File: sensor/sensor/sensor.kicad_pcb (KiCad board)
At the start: 2 copper layers, 39 parts, among them J1 RJ12_Shielded, J2 Conn_01x04, J3 Conn_01x06, J4 Conn_01x05, J5 Conn_01x05, J8 RJ12_Shielded, J9 Conn_01x06, SW5 SW_Coded_SH-7050, U1 PCA9615DP, U2 LTC4316, U5 TPS73101DBV

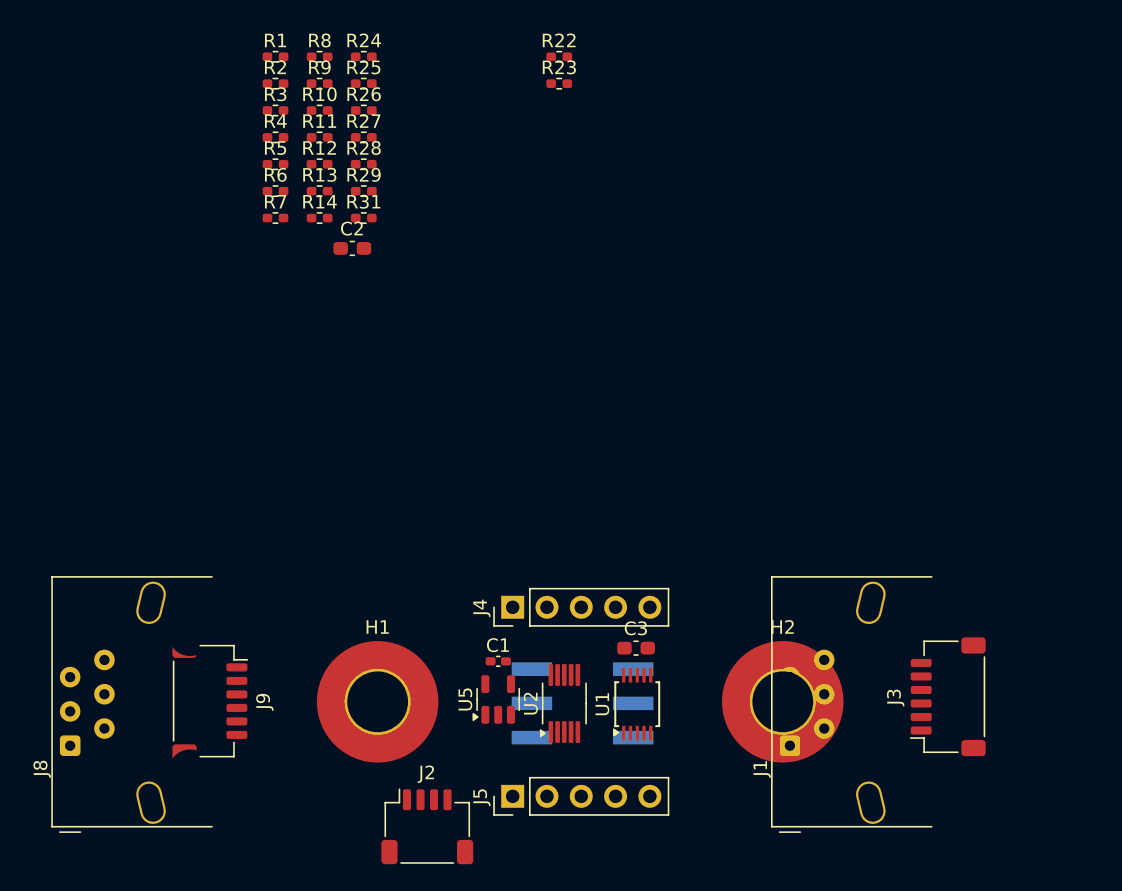
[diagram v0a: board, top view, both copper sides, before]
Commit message: finished main sensor board
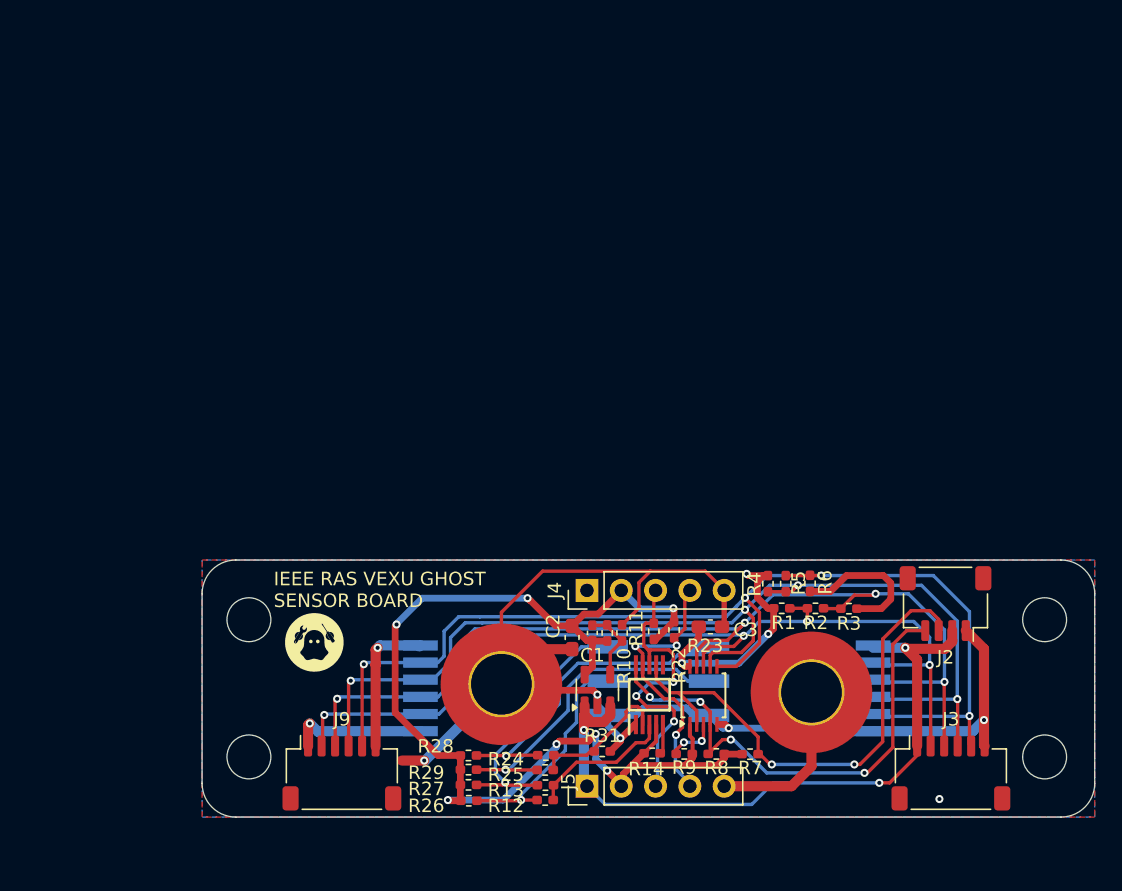
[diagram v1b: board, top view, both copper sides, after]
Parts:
- removed J8: RJ12_Shielded, RJ12_Pin_Connector:RJ12_Pin_Connector
- removed U2: LTC4316, Package_SO:MSOP-10_3x3mm_P0.5mm
- added G***: LOGO, LOGO, F.Cu at (110.3, 105.6)
- added G***: LOGO, LOGO, B.Cu at (110.7, 102.8)
- added G***: LOGO, LOGO, B.Cu at (114.8, 101.9)
- added IC1: LTC4316CMS#TRPBF, LTC4316CMS:SOP50P490X110-10N, F.Cu at (135.1, 109.5)
- added J6: GDLX-SMT-N-66, GDLX-SMT-N-66:GDLXSMTN66, B.Cu at (107.9, 109.0)
- J1: value RJ12_Shielded -> GDLX-SMT-N-66; footprint RJ12_Pin_Connector:RJ12_Pin_Connector -> GDLX-SMT-N-66:GDLXSMTN66; moved to B.Cu
- moved R8 59.4 mm to (140.1, 113.9), turned to 180 degrees
- moved R9 56.5 mm to (137.7, 113.9), turned to 180 degrees
- moved R3 56.2 mm to (149.9, 103.1)
- moved R2 55.8 mm to (147.4, 103.1), turned to 180 degrees
- moved R1 55.4 mm to (144.9, 103.1)
- moved R24 53.4 mm to (127.5, 114.0)
- moved R7 53.0 mm to (142.6, 113.9)
- moved R25 52.6 mm to (127.4, 115.0)
- moved R26 51.7 mm to (121.8, 117.3)
- moved R12 50.0 mm to (127.4, 117.3)
- moved R4 49.2 mm to (143.9, 101.2), turned to -90 degrees
- moved R6 49.1 mm to (147.0, 101.2), turned to -90 degrees
- moved R5 48.9 mm to (145.2, 101.2), turned to -90 degrees
- moved R27 48.6 mm to (121.7, 116.2)
- moved R13 47.1 mm to (127.4, 116.2)
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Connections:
- R14 pad 1: +3.3V -> Net-(IC1-ENABLE)
- R14 pad 2: Net-(U2-ENABLE) -> +3.3V
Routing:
- net GND: track 0.00 -> 137.8 mm, vias 0 -> 6
- net +3.3V: track 0.00 -> 85.2 mm, vias 0 -> 7
- net Net-(J3-Pin_5): track 0.00 -> 83.5 mm, vias 0 -> 4
- net Net-(J3-Pin_4): track 0.00 -> 79.9 mm, vias 0 -> 4
- net +5V: track 0.00 -> 79.6 mm, vias 0 -> 7
- net Net-(J3-Pin_3): track 0.00 -> 78.3 mm, vias 0 -> 4
- net Net-(J3-Pin_2): track 0.00 -> 71.6 mm, vias 0 -> 4
- net Net-(IC1-SDAIN): track 0.00 -> 38.5 mm, vias 0 -> 2
- net Net-(IC1-SCLIN): track 0.00 -> 37.3 mm, vias 0 -> 4
- net Net-(R25-Pad1): track 0.00 -> 24.0 mm, vias 0 -> 1
- net Net-(R24-Pad1): track 0.00 -> 23.9 mm, vias 0 -> 1
- net /Sensors/sda: track 0.00 -> 23.1 mm, vias 0 -> 3
- net /Sensors/scl: track 0.00 -> 20.9 mm, vias 0 -> 3
- net Net-(R13-Pad1): track 0.00 -> 19.6 mm, vias 0 -> 1
- net Net-(R12-Pad1): track 0.00 -> 16.8 mm, vias 0 -> 1
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- added copper zone on B.Cu, net +5V
- added copper zone on F.Cu, net GND
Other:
- board outline added: 66.1 x 19 mm
- board text added: "ALLEN A KARMA. M ANDREW K JENNY C"
- board text added: "IEEE RAS VEXU GHOST SENSOR BOARD"
